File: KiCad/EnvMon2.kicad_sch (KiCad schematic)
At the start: 35 parts, among them J1 USB-C, J2 DC, J3 TEMP, M1 OLED1.5-RGB, SW1 SW_Push, SW2 SW_Push, SW3 SW_Push, U1 LMR16006+FB, U2 SCD41, U3 FT231XQ, U4 ESP32-PICO-MINI-02, U5 QR

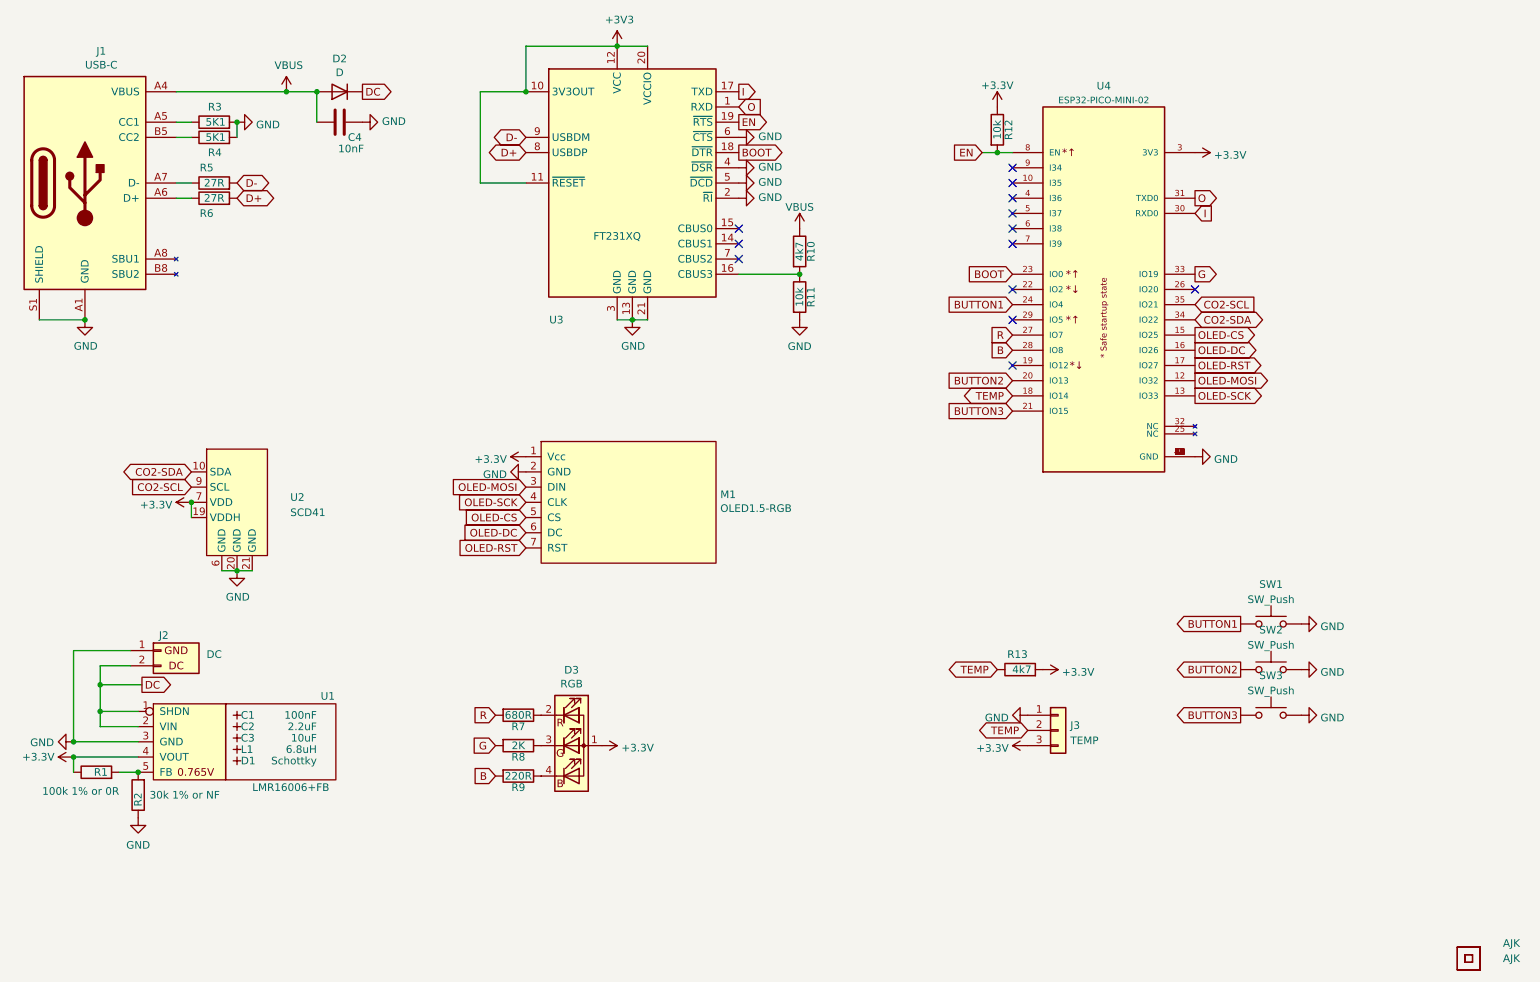
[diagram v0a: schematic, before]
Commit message: Some PCB rework in progress
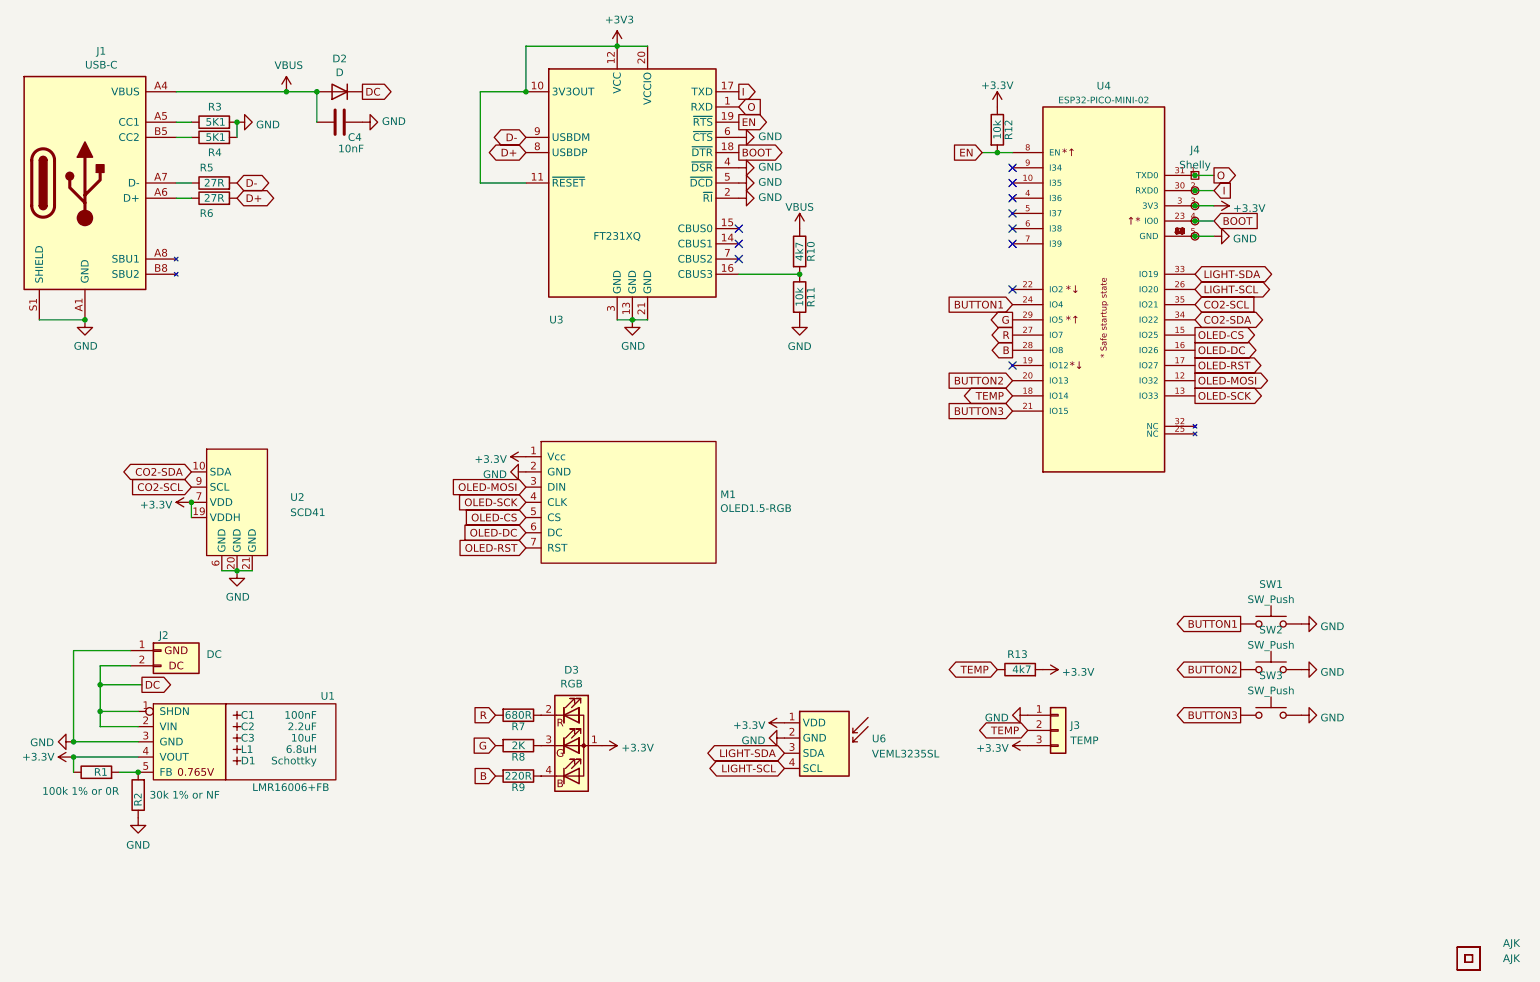
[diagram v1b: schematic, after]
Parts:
- added J4: Shelly, RevK:Shelly, symbol RevK:Shelly
- added U6: VEML3235SL, RevK:VEML3235SL, symbol RevK:VEML3235SL
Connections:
- net +3V3: now also J4.3 (3V3), U6.1 (VDD)
- net BOOT: now also J4.4 (Rx)
- net G: now also U4.29 (IO5); no longer U4.33 (IO19)
- net GND: now also J4.5 (Tx), U6.2 (GND)
- net I: now also J4.2 (0)
- net O: now also J4.1 (GND)
- net LIGHT-SCL: now reaches U4.26 (IO20)
- net LIGHT-SCL: now also U6.4 (SCL)
- new net LIGHT-SDA: U4.33 (IO19), U6.3 (SDA)
- no-connect marks 13 -> 11

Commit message: Revised PCB for light sensor
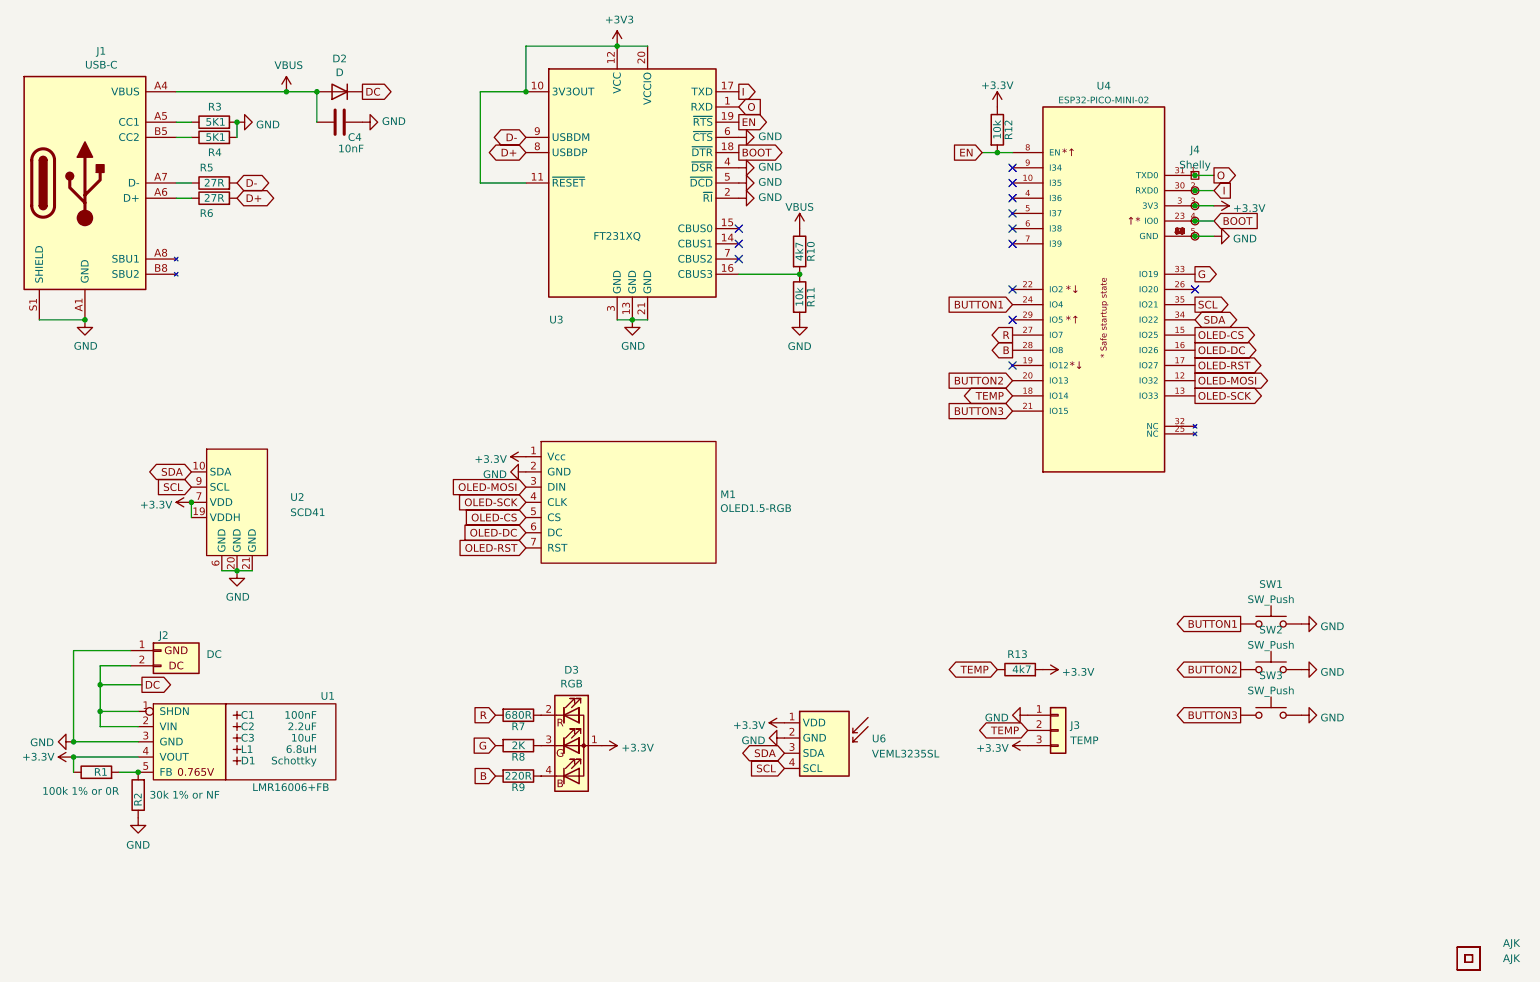
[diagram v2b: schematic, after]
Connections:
- net G: now also U4.33 (IO19); no longer U4.29 (IO5)
- net CO2-SCL renamed SCL
- net SCL: now also U6.4 (SCL)
- net CO2-SDA renamed SDA
- net SDA: now also U6.3 (SDA)
- net LIGHT-SCL: no longer names the net of U4.26 (IO20)
- net LIGHT-SCL: no longer U6.4 (SCL)
- removed net LIGHT-SDA: U4.33 (IO19), U6.3 (SDA)
- no-connect marks 11 -> 13
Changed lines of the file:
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@@
   )
   (no_connect (at 149.86 55.88))
+  (no_connect (at 195.58 66.04))
+  (no_connect (at 226.06 60.96))
   (no_connect (at 149.86 50.8))
   (no_connect (at 149.86 53.34))
@@
     )
   )
-  (global_label "LIGHT-SCL" (shape bidirectional) (at 226.06 60.96 0) (fields_autoplaced)
-    (effects (font (size 1.27 1.27)) (justify left))
-    (property "Intersheet References" "${INTERSHEET_REFS}" (id 0) (at 238.6652 61.0394 0)
-      (effects (font (size 1.27 1.27)) (justify left) hide)
-    )
-  )
   (global_label "TEMP" (shape bidirectional) (at 198.12 134.62 180) (fields_autoplaced)
     (effects (font (size 1.27 1.27)) (justify right))
@@
     )
   )
-  (global_label "CO2-SCL" (shape input) (at 226.06 63.5 0) (fields_autoplaced)
-    (effects (font (size 1.27 1.27)) (justify left))
-    (property "Intersheet References" "${INTERSHEET_REFS}" (id 0) (at 274.955 184.785 0)
-      (effects (font (size 1.27 1.27)) hide)
+  (global_label "SCL" (shape output) (at 226.06 63.5 0) (fields_autoplaced)
+    (effects (font (size 1.27 1.27)) (justify left))
+    (property "Intersheet References" "${INTERSHEET_REFS}" (id 0) (at 231.8918 63.4206 0)
+      (effects (font (size 1.27 1.27)) (justify left) hide)
     )
   )
@@
     )
   )
-  (global_label "LIGHT-SDA" (shape bidirectional) (at 157.48 138.43 180) (fields_autoplaced)
-    (effects (font (size 1.27 1.27)) (justify right))
-    (property "Intersheet References" "${INTERSHEET_REFS}" (id 0) (at 144.8144 138.3506 0)
+  (global_label "SDA" (shape bidirectional) (at 157.48 138.43 180) (fields_autoplaced)
+    (effects (font (size 1.27 1.27)) (justify right))
+    (property "Intersheet References" "${INTERSHEET_REFS}" (id 0) (at 151.5877 138.3506 0)
       (effects (font (size 1.27 1.27)) (justify right) hide)
     )
@@
     )
   )
-  (global_label "CO2-SCL" (shape input) (at 58.42 93.98 180) (fields_autoplaced)
-    (effects (font (size 1.27 1.27)) (justify right))
-    (property "Intersheet References" "${INTERSHEET_REFS}" (id 0) (at 9.525 -27.305 0)
-      (effects (font (size 1.27 1.27)) hide)
-    )
-  )
-  (global_label "LIGHT-SCL" (shape bidirectional) (at 157.48 140.97 180) (fields_autoplaced)
-    (effects (font (size 1.27 1.27)) (justify right))
-    (property "Intersheet References" "${INTERSHEET_REFS}" (id 0) (at 144.8748 140.8906 0)
+  (global_label "SCL" (shape input) (at 58.42 93.98 180) (fields_autoplaced)
+    (effects (font (size 1.27 1.27)) (justify right))
+    (property "Intersheet References" "${INTERSHEET_REFS}" (id 0) (at 52.5882 93.9006 0)
+      (effects (font (size 1.27 1.27)) (justify right) hide)
+    )
+  )
+  (global_label "SCL" (shape input) (at 157.48 140.97 180) (fields_autoplaced)
+    (effects (font (size 1.27 1.27)) (justify right))
+    (property "Intersheet References" "${INTERSHEET_REFS}" (id 0) (at 151.6482 140.8906 0)
       (effects (font (size 1.27 1.27)) (justify right) hide)
     )
@@
     )
   )
-  (global_label "G" (shape output) (at 195.58 66.04 180) (fields_autoplaced)
-    (effects (font (size 1.27 1.27)) (justify right))
-    (property "Intersheet References" "${INTERSHEET_REFS}" (id 0) (at 191.9858 66.1194 0)
-      (effects (font (size 1.27 1.27)) (justify right) hide)
+  (global_label "G" (shape output) (at 226.06 58.42 0) (fields_autoplaced)
+    (effects (font (size 1.27 1.27)) (justify left))
+    (property "Intersheet References" "${INTERSHEET_REFS}" (id 0) (at 229.6542 58.3406 0)
+      (effects (font (size 1.27 1.27)) (justify left) hide)
     )
   )
@@
     )
   )
-  (global_label "CO2-SDA" (shape bidirectional) (at 226.06 66.04 0) (fields_autoplaced)
-    (effects (font (size 1.27 1.27)) (justify left))
-    (property "Intersheet References" "${INTERSHEET_REFS}" (id 0) (at 237.3347 65.9606 0)
+  (global_label "SDA" (shape bidirectional) (at 226.06 66.04 0) (fields_autoplaced)
+    (effects (font (size 1.27 1.27)) (justify left))
+    (property "Intersheet References" "${INTERSHEET_REFS}" (id 0) (at 231.9523 65.9606 0)
       (effects (font (size 1.27 1.27)) (justify left) hide)
     )
@@
     )
   )
-  (global_label "LIGHT-SDA" (shape bidirectional) (at 226.06 58.42 0) (fields_autoplaced)
-    (effects (font (size 1.27 1.27)) (justify left))
-    (property "Intersheet References" "${INTERSHEET_REFS}" (id 0) (at 238.7256 58.4994 0)
-      (effects (font (size 1.27 1.27)) (justify left) hide)
-    )
-  )
-  (global_label "CO2-SDA" (shape bidirectional) (at 58.42 91.44 180) (fields_autoplaced)
-    (effects (font (size 1.27 1.27)) (justify right))
-    (property "Intersheet References" "${INTERSHEET_REFS}" (id 0) (at 47.1453 91.3606 0)
-      (effects (font (size 1.27 1.27)) (justify right) hide)
-    )
+  (global_label "SDA" (shape bidirectional) (at 58.42 91.44 180) (fields_autoplaced)
+    (effects (font (size 1.27 1.27)) (justify right))
+    (property "Intersheet References" "${INTERSHEET_REFS}" (id 0) (at 52.5277 91.3606 0)
+      (effects (font (size 1.27 1.27)) (justify right) hide)
+    )
